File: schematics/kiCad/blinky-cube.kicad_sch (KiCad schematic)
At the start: 25 parts, among them J1 Screw_Terminal_01x03, J2 Screw_Terminal_01x03, J3 Screw_Terminal_01x03, J4 Screw_Terminal_01x03, SW1 SW_Push, U1 Pico, U2 LM4040LP-3, U3 BZX84C3V3, U4 BZX84C3V3, U5 BZX84C3V3

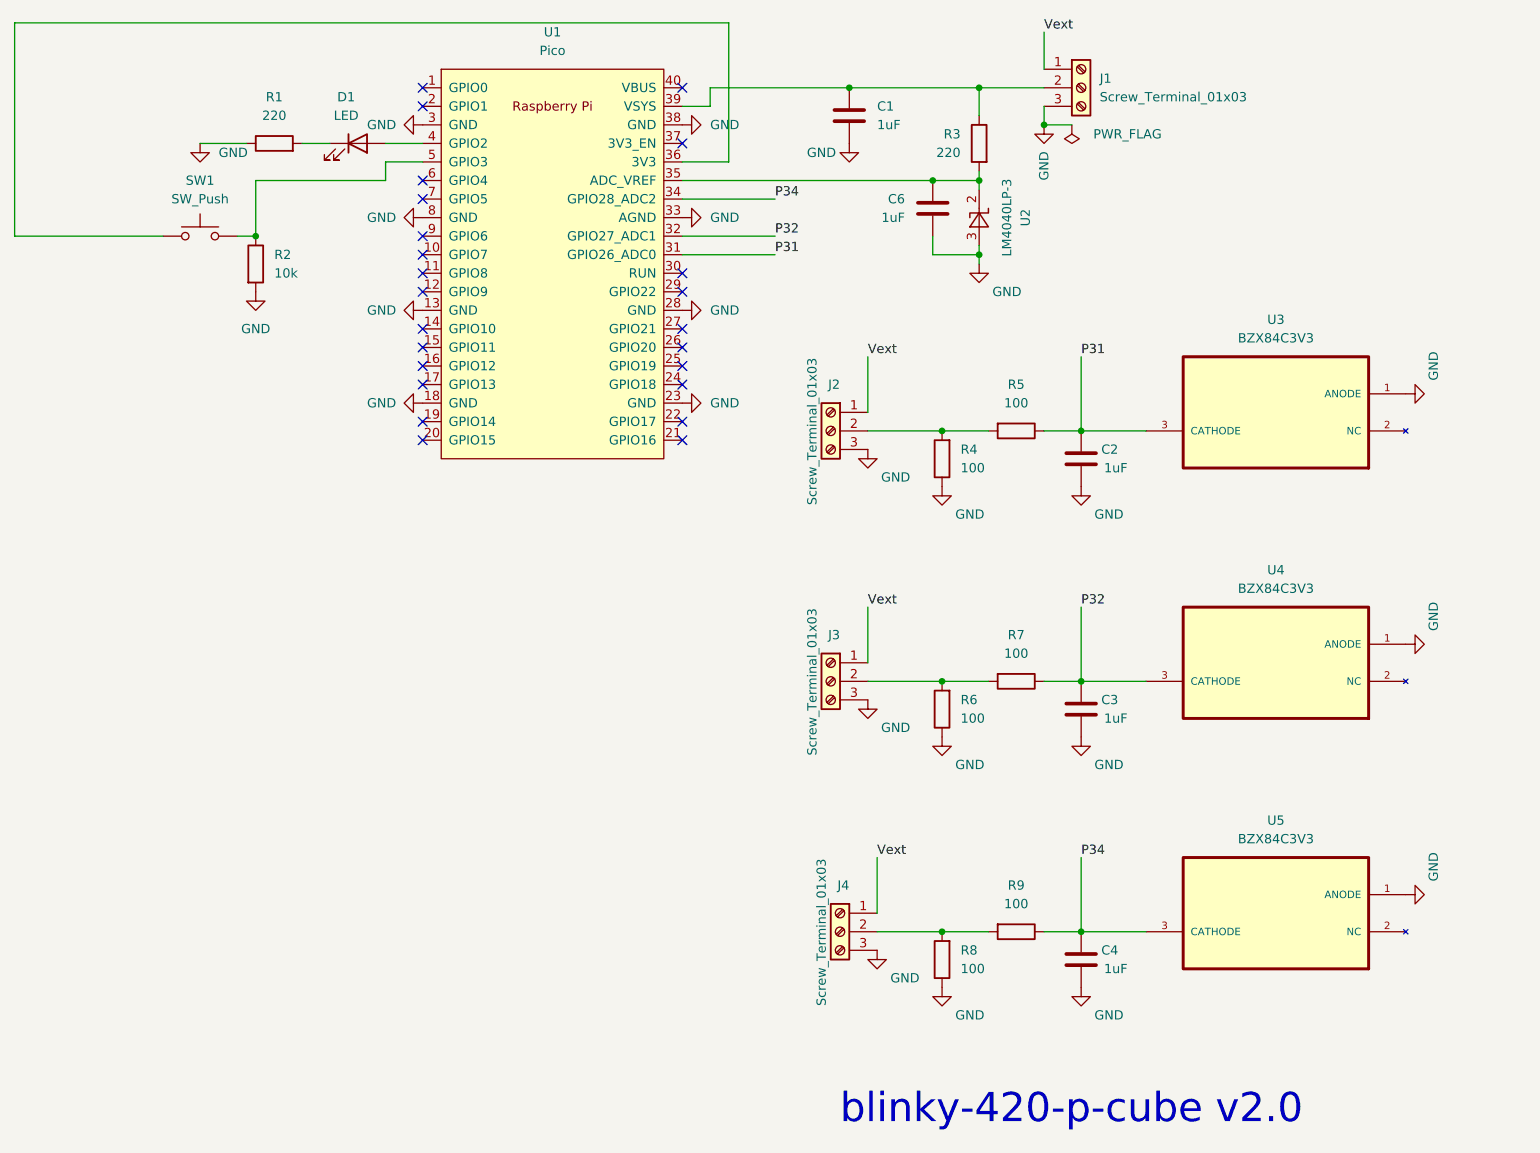
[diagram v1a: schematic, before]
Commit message: layout complete
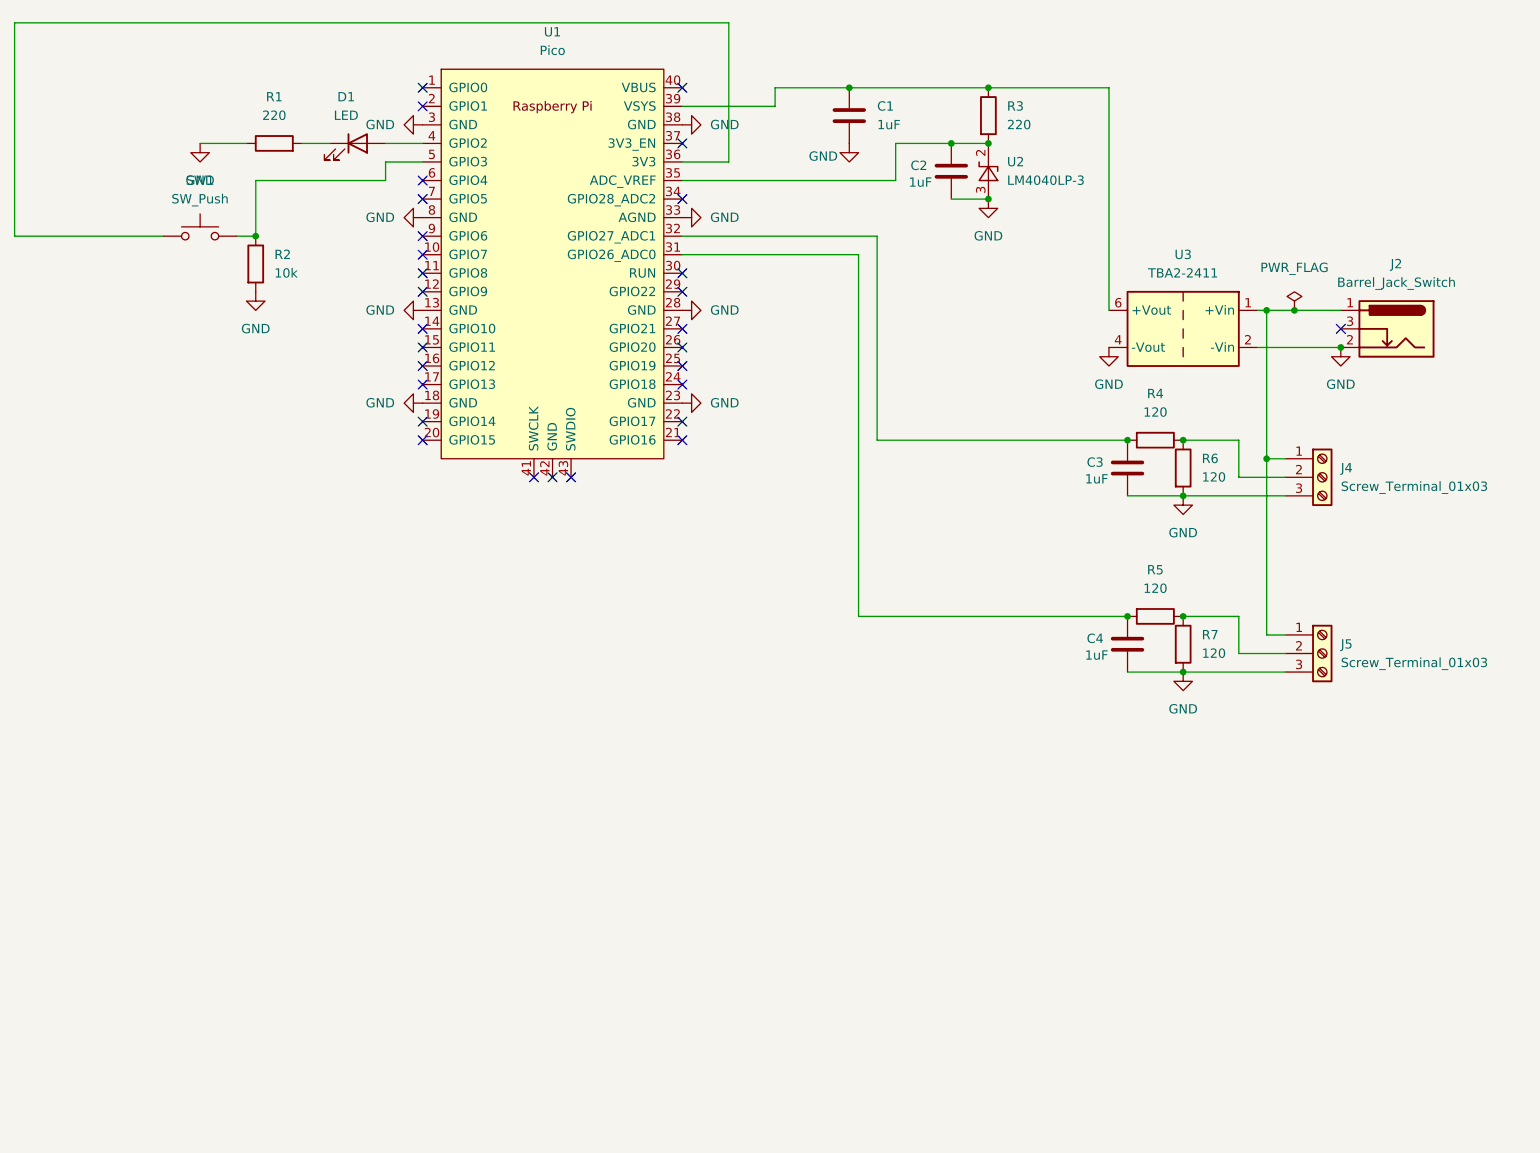
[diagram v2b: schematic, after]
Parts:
- removed C6: 1uF, Capacitor_SMD:C_1206_3216Metric_Pad1.33x1.80mm_HandSolder, symbol Device:C
- removed J1, J2, J3: Screw_Terminal_01x03, TerminalBlock:TerminalBlock_bornier-3_P5.08mm, symbol Connector:Screw_Terminal_01x03
- removed R8, R9: 100, Resistor_SMD:R_1206_3216Metric_Pad1.30x1.75mm_HandSolder, symbol Device:R
- removed U3, U4, U5: BZX84C3V3, BZX84C3V3:SOT91P240X110-3N, symbol BZX84C3V3:BZX84C3V3
- added J2: Barrel_Jack_Switch, Connector_BarrelJack:BarrelJack_Horizontal, symbol Connector:Barrel_Jack_Switch
- added J5: Screw_Terminal_01x03, TerminalBlock_Phoenix:TerminalBlock_Phoenix_MKDS-3-3-5.08_1x03_P5.08mm_Horizontal, symbol Connector:Screw_Terminal_01x03
- added U3: TBA2-2411, Converter_DCDC:Converter_DCDC_TRACO_TBA2-xxxx_Single_THT, symbol Converter_DCDC:TBA2-2411
- C1, C2, C3, C4: footprint Capacitor_SMD:C_1206_3216Metric_Pad1.33x1.80mm_HandSolder -> Capacitor_THT:C_Disc_D4.7mm_W2.5mm_P5.00mm
- J4: footprint TerminalBlock:TerminalBlock_bornier-3_P5.08mm -> TerminalBlock_Phoenix:TerminalBlock_Phoenix_MKDS-3-3-5.08_1x03_P5.08mm_Horizontal
- R1, R2, R3: footprint Resistor_SMD:R_1206_3216Metric_Pad1.30x1.75mm_HandSolder -> Resistor_THT:R_Axial_DIN0207_L6.3mm_D2.5mm_P7.62mm_Horizontal
- R4, R5, R6, R7: value 100 -> 120; footprint Resistor_SMD:R_1206_3216Metric_Pad1.30x1.75mm_HandSolder -> Resistor_THT:R_Axial_DIN0207_L6.3mm_D2.5mm_P7.62mm_Horizontal
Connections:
- net GND: now also R6.2, R7.2, J2.2, J5.3 (Pin_3), U3.2 (-Vin), U3.4 (-Vout); no longer R4.1, R6.1
- net at C1.1, R3.1, U1.39 (VSYS): now also U3.6 (+Vout)
- net at R3.2, U1.35 (ADC_VREF), U2.2 (K): now also C2.1
- net at R5.2: now also C4.1, U1.31 (GPIO26_ADC0); no longer R4.2
- net at J4.2 (Pin_2): now also R4.1, R6.1
- removed net P31: C2.1, R5.1, U1.31 (GPIO26_ADC0)
- net P32: no longer names the net of C3.1, U1.32 (GPIO27_ADC1)
- net P32: now also R4.2; no longer R7.1
- net P34: no longer names the net of U1.34 (GPIO28_ADC2)
- net P34: no longer C4.1
- net Vext: no longer names the net of J4.1 (Pin_1)
- net Vext: now also J2.1, J5.1 (Pin_1), U3.1 (+Vin)
- new net: J5.2 (Pin_2), R5.1, R7.1
- no-connect marks 24 -> 29
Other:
- note removed: "blinky-420-p-cube v2.0"
